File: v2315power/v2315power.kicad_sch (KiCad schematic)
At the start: 12 parts, among them J1 Screw_Terminal_01x10, J2 Screw_Terminal_01x01, Q1 2N3904

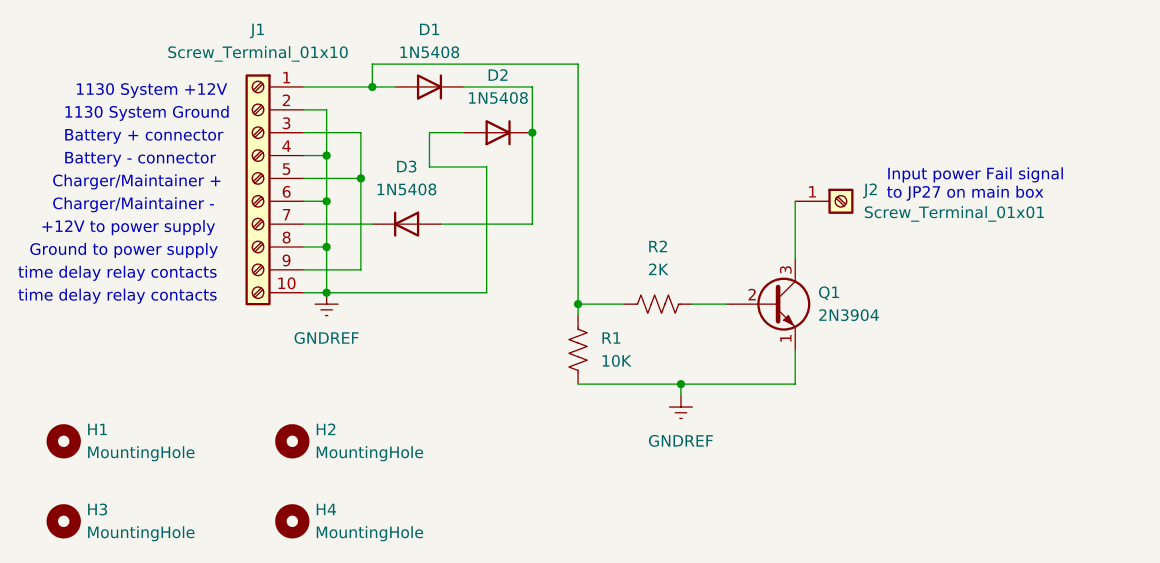
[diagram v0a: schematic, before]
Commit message: Update after testing
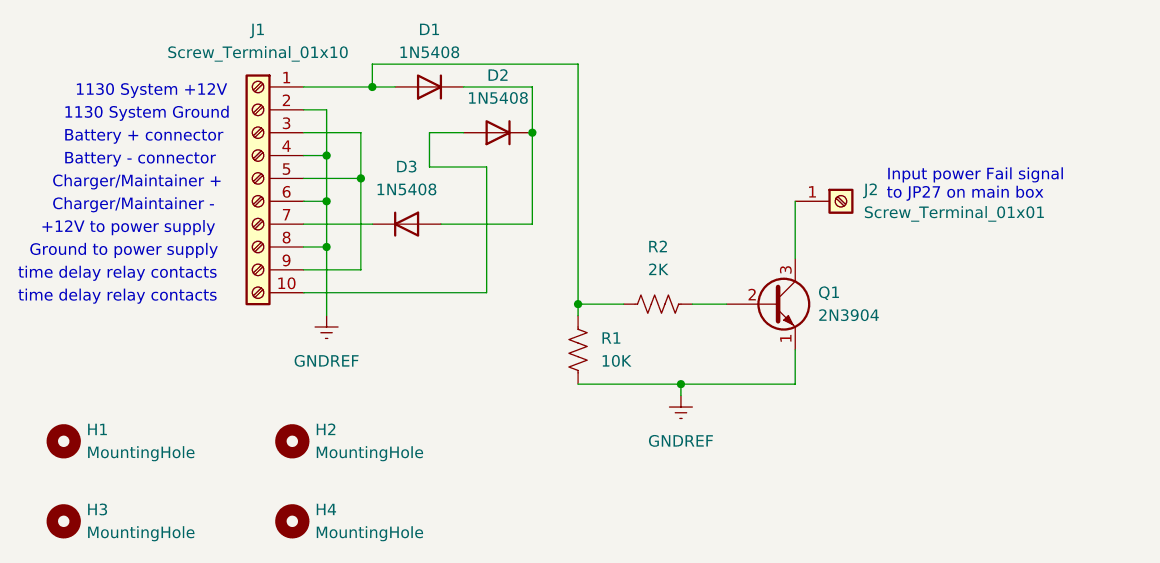
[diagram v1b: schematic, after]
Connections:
- net GNDREF: no longer D2.2 (A), J1.10 (Pin_10)
- new net: D2.2 (A), J1.10 (Pin_10)
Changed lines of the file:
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@@
   (junction (at 54.61 50.8) (diameter 0) (color 0 0 0 0)
   )
-  (junction (at 54.61 60.96) (diameter 0) (color 0 0 0 0)
-  )
   (junction (at 93.98 71.12) (diameter 0) (color 0 0 0 0)
   )
@@
     (stroke (width 0) (type default))
   )
-  (wire (pts (xy 54.61 60.96) (xy 54.61 55.88))
+  (wire (pts (xy 54.61 63.5) (xy 54.61 55.88))
     (stroke (width 0) (type default))
   )
@@
     (stroke (width 0) (type default))
   )
-  (wire (pts (xy 54.61 60.96) (xy 72.39 60.96))
-    (stroke (width 0) (type default))
-  )
   (wire (pts (xy 82.55 35.56) (xy 82.55 62.23))
     (stroke (width 0) (type default))
@@
     (stroke (width 0) (type default))
   )
-  (wire (pts (xy 52.07 60.96) (xy 54.61 60.96))
+  (wire (pts (xy 52.07 60.96) (xy 72.39 60.96))
     (stroke (width 0) (type default))
   )
@@
     )
   )
-  (symbol (lib_id "power:GNDREF") (at 54.61 60.96 0) (unit 1)
-    (in_bom yes) (on_board yes) (dnp no) (fields_autoplaced)
-    (property "Reference" "#PWR01" (at 54.61 67.31 0)
-      (effects (font (size 1.27 1.27)) hide)
-    )
-    (property "Value" "GNDREF" (at 54.61 66.04 0)
+  (symbol (lib_id "power:GNDREF") (at 54.61 63.5 0) (unit 1)
+    (in_bom yes) (on_board yes) (dnp no) (fields_autoplaced)
+    (property "Reference" "#PWR01" (at 54.61 69.85 0)
+      (effects (font (size 1.27 1.27)) hide)
+    )
+    (property "Value" "GNDREF" (at 54.61 68.58 0)
       (effects (font (size 1.27 1.27)))
     )
-    (property "Footprint" "" (at 54.61 60.96 0)
-      (effects (font (size 1.27 1.27)) hide)
-    )
-    (property "Datasheet" "" (at 54.61 60.96 0)
-      (effects (font (size 1.27 1.27)) hide)
-    )
+    (property "Footprint" "" (at 54.61 63.5 0)
+      (effects (font (size 1.27 1.27)) hide)
+    )
+    (property "Datasheet" "" (at 54.61 63.5 0)
+      (effects (font (size 1.27 1.27)) hide)
+    )
